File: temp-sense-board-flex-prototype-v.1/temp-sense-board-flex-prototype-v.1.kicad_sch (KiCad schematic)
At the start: 11 parts, among them J10 84952-5, J11 0015388040, J2 512810598, J8 GHR-04V-S1, J9 SM04B-GHS-TB1, U1 TMP1075D, U2 TMP1075D, U3 TMP1075D

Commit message: more connectors w footprints
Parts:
- J10: footprint (none) -> Connector_FFC-FPC:TE_1-84952-5_1x15-1MP_P1.0mm_Horizontal
- J8: Digikey URL https://www.jst-mfg.com/product/pdf/eng/eGH.pdf -> https://www.digikey.com/en/products/detail/jst-sales-americ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
- J9: footprint (none) -> Connector_JST:JST_GH_SM04B-GHS-TB_1x04-1MP_P1.25mm_Horizontal
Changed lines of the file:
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@@
 			)
 		)
-		(property "Footprint" ""
+		(property "Footprint" "Connector_FFC-FPC:TE_1-84952-5_1x15-1MP_P1.0mm_Horizontal"
 			(at 74.93 99.06 0)
 			(hide yes)
@@
 			)
 		)
-		(property "Footprint" ""
+		(property "Footprint" "Connector_JST:JST_GH_SM04B-GHS-TB_1x04-1MP_P1.25mm_Horizontal"
 			(at 74.93 115.57 0)
 			(hide yes)
@@
 			)
 		)
-		(property "Datasheet" ""
+		(property "Datasheet" "https://www.jst-mfg.com/product/pdf/eng/eGH.pdf"
 			(at 74.93 130.81 0)
 			(hide yes)
@@
 			)
 		)
-		(property "Digikey URL" "https://www.jst-mfg.com/product/pdf/eng/eGH.pdf"
+		(property "Digikey URL" "https://www.digikey.com/en/products/detail/jst-sales-america-inc/GHR-04V-S/807816?msockid=15685f35b86e654907ab4928b9226472"
 			(at 74.93 130.81 0)
 			(hide yes)

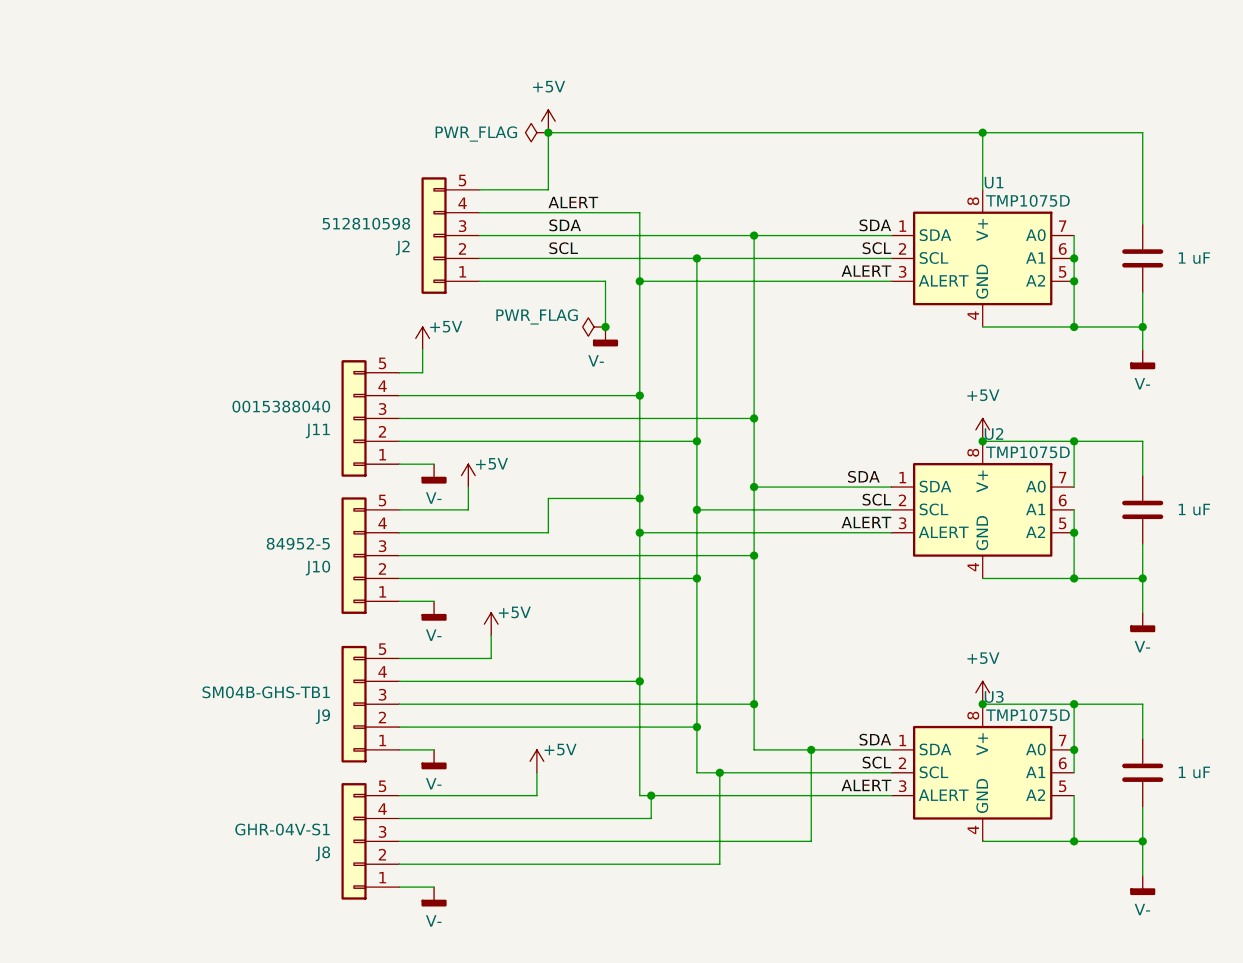
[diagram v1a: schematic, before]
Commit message: schematic is finished; layout is not
-added footprints to fs library
-finalized schematic
-did a veeery rough layout not complete jiust here tonight
-yay eh someone give comments
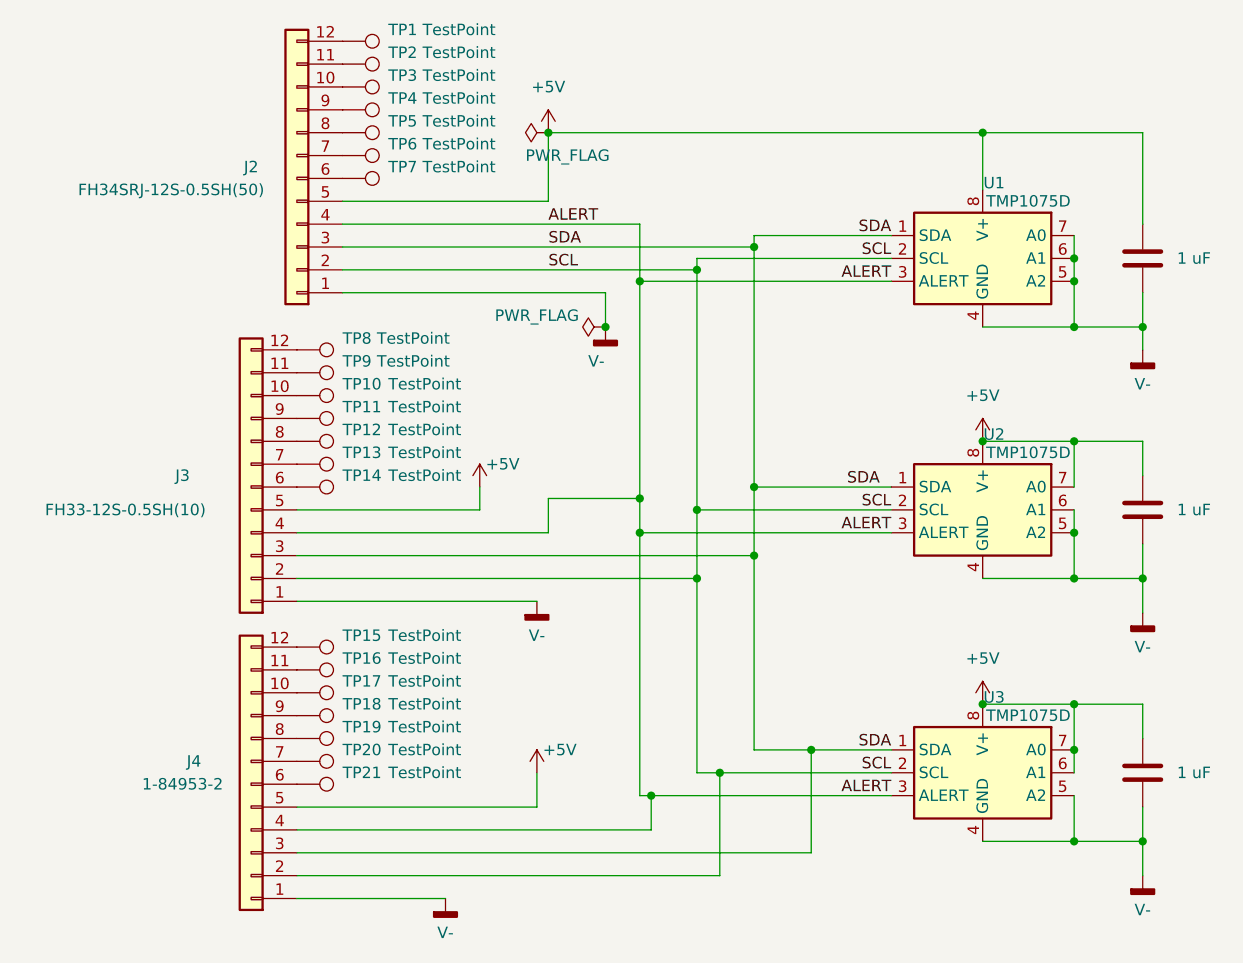
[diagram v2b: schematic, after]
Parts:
- removed J10: 84952-5, Connector_FFC-FPC:TE_1-84952-5_1x15-1MP_P1.0mm_Horizontal, symbol Connector_Generic:Conn_01x05
- removed J11: 0015388040, symbol Connector_Generic:Conn_01x05
- removed J2: 512810598, FS_4_Footprint_Library:512810598, symbol Connector_Generic:Conn_01x05
- removed J8: GHR-04V-S1, symbol Connector_Generic:Conn_01x05
- removed J9: SM04B-GHS-TB1, Connector_JST:JST_GH_SM04B-GHS-TB_1x04-1MP_P1.25mm_Horizontal, symbol Connector_Generic:Conn_01x05
- added J2: FH34SRJ-12S-0.5SH(50), formula_slug_footprint_library:CONN12x1_FH34SRJ-12S-0.5SH50_HIR, symbol Connector_Generic:Conn_01x12
- added J3: FH33-12S-0.5SH(10), formula_slug_footprint_library:CONN_FH33-12S-0.5SH10_HIR, symbol Connector_Generic:Conn_01x12
- added J4: 1-84953-2, formula_slug_footprint_library:CON12_SMT-RA_FCC-FPC2, symbol Connector_Generic:Conn_01x12
- added TP1, TP10, TP11, TP12, TP13, TP14, TP15, TP16, TP17, TP18, TP19, TP2, TP20, TP21, TP3, TP4, TP5, TP6, TP7, TP8, TP9: TestPoint, TestPoint:TestPoint_Pad_D1.0mm, symbol Connector:TestPoint
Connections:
- net +5V: now also J2.5 (Pin_5), J3.5 (Pin_5), J4.5 (Pin_5)
- net ALERT: now also J2.4 (Pin_4), J3.4 (Pin_4), J4.4 (Pin_4)
- net SCL: now also J2.2 (Pin_2), J3.2 (Pin_2), J4.2 (Pin_2)
- net SDA: now also J2.3 (Pin_3), J3.3 (Pin_3), J4.3 (Pin_3)
- net V-: now also J2.1 (Pin_1), J3.1 (Pin_1), J4.1 (Pin_1)
- new net: J4.6 (Pin_6), TP21.1
- new net: J2.10 (Pin_10), TP3.1
- new net: J3.12 (Pin_12), TP8.1
- new net: J2.8 (Pin_8), TP5.1
- new net: J4.10 (Pin_10), TP17.1
- new net: J4.11 (Pin_11), TP16.1
- new net: J4.12 (Pin_12), TP15.1
- new net: J4.7 (Pin_7), TP20.1
- new net: J4.8 (Pin_8), TP19.1
- new net: J4.9 (Pin_9), TP18.1
- new net: J3.10 (Pin_10), TP10.1
- new net: J3.11 (Pin_11), TP9.1
- new net: J3.6 (Pin_6), TP14.1
- new net: J3.7 (Pin_7), TP13.1
- new net: J3.8 (Pin_8), TP12.1
- new net: J3.9 (Pin_9), TP11.1
- new net: J2.6 (Pin_6), TP7.1
- new net: J2.9 (Pin_9), TP4.1
- new net: J2.11 (Pin_11), TP2.1
- new net: J2.12 (Pin_12), TP1.1
- new net: J2.7 (Pin_7), TP6.1

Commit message: first trace thing done
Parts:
- J4: footprint formula_slug_footprint_library:CON12_SMT-RA_FCC-FPC2 -> formula_slug_footprint_library:FPC-12PIN-CABLE-1mm-0.71mm
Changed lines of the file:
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@@
 			)
 		)
-		(property "Footprint" "formula_slug_footprint_library:CON12_SMT-RA_FCC-FPC2"
+		(property "Footprint" "formula_slug_footprint_library:FPC-12PIN-CABLE-1mm-0.71mm"
 			(at 63.5 124.46 0)
 			(hide yes)
